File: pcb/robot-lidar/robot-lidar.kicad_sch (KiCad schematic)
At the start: 7 parts, among them J2 YLIDAR X4, J3 Jack-DC, U1 STM32F429VETx, U2 LM317-3.3_SOT-223

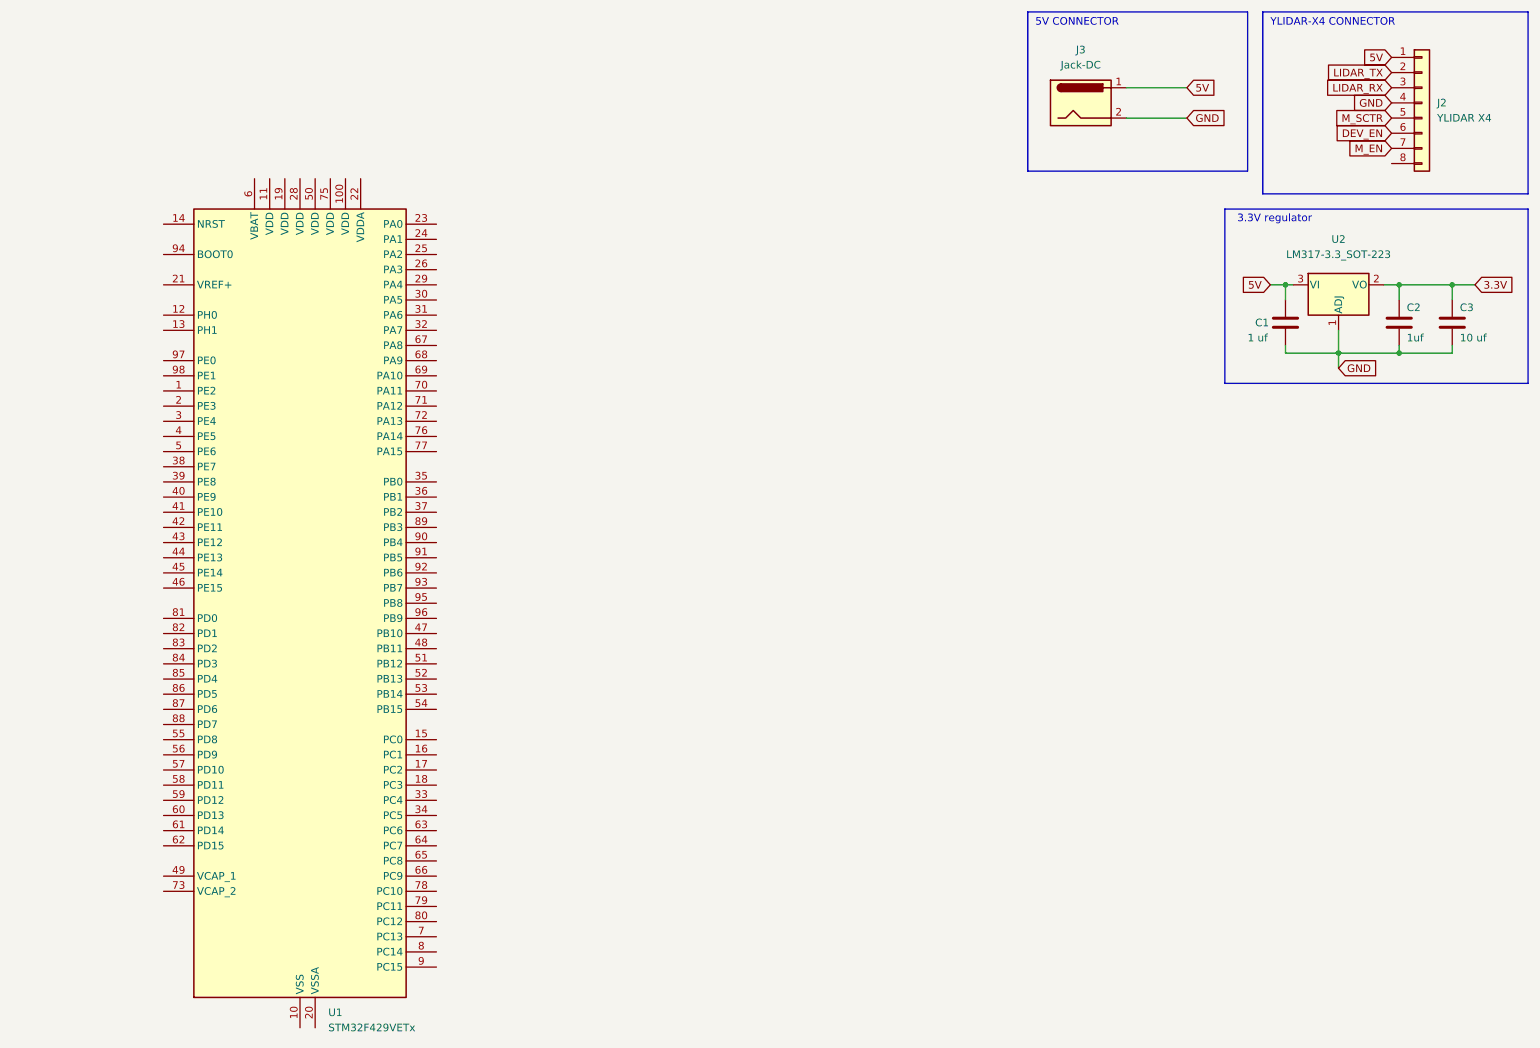
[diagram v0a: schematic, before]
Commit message: add gyro
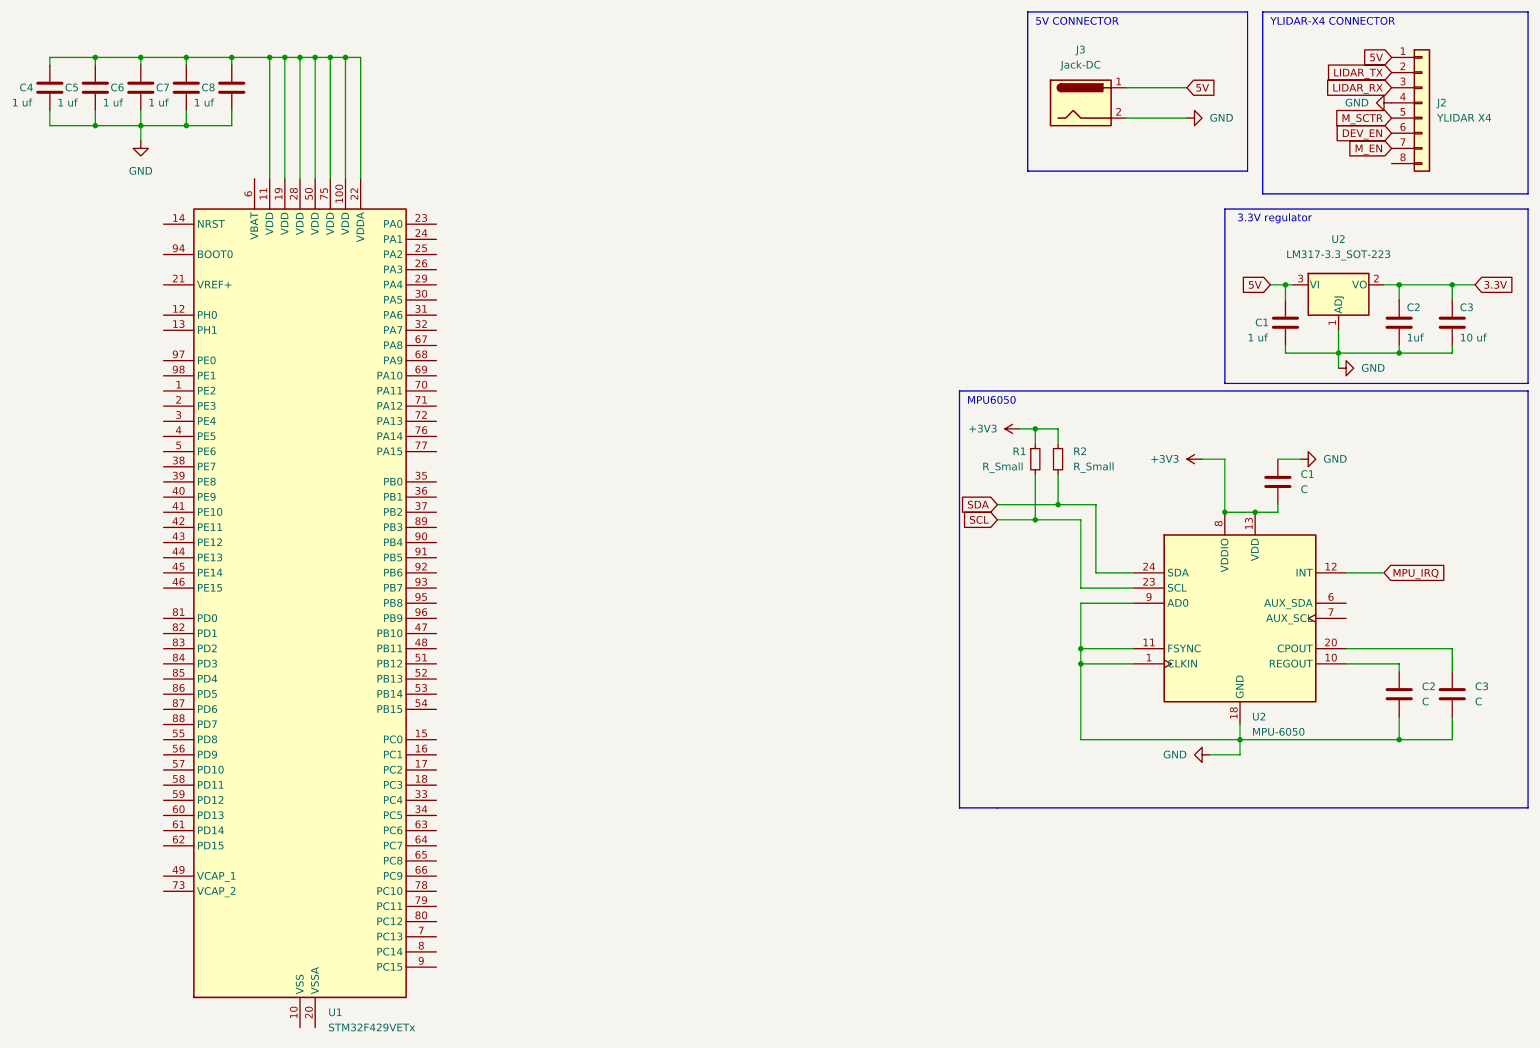
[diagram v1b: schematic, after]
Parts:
- added C1, C2, C3: C, Capacitor_SMD:C_0603_1608Metric, symbol Device:C
- added C4, C5, C6, C7, C8: 1 uf, Capacitor_SMD:C_0603_1608Metric, symbol Device:C
- added R1, R2: R_Small, Resistor_SMD:R_0603_1608Metric, symbol Device:R_Small
- added U2: MPU-6050, Sensor_Motion:InvenSense_QFN-24_4x4mm_P0.5mm, symbol Sensor_Motion:MPU-6050
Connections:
- net GND: now also C1.1, C2.2, C3.2, C4.2, C5.2, C6.2, C7.2, C8.2, U2.1 (CLKIN), U2.11 (FSYNC), U2.18 (GND), U2.9 (AD0)
- net at U1.100 (VDD): now also U1.11 (VDD), U1.19 (VDD), U1.22 (VDDA), U1.28 (VDD), U1.50 (VDD), U1.75 (VDD), C4.1, C5.1, C6.1, C7.1, C8.1
- new net: C3.1, U2.20 (CPOUT)
- new net: C2.1, U2.10 (REGOUT)
- new net +3V3: C1.2, R1.1, R2.1, U2.13 (VDD), U2.8 (VDDIO)
- new net MPU_IRQ: U2.12 (INT)
- new net SCL: R1.2, U2.23 (SCL)
- new net SDA: R2.2, U2.24 (SDA)
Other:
- note added: "MPU6050"
